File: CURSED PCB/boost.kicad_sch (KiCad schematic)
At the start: 6 parts, among them U11 TPS61046YFFR

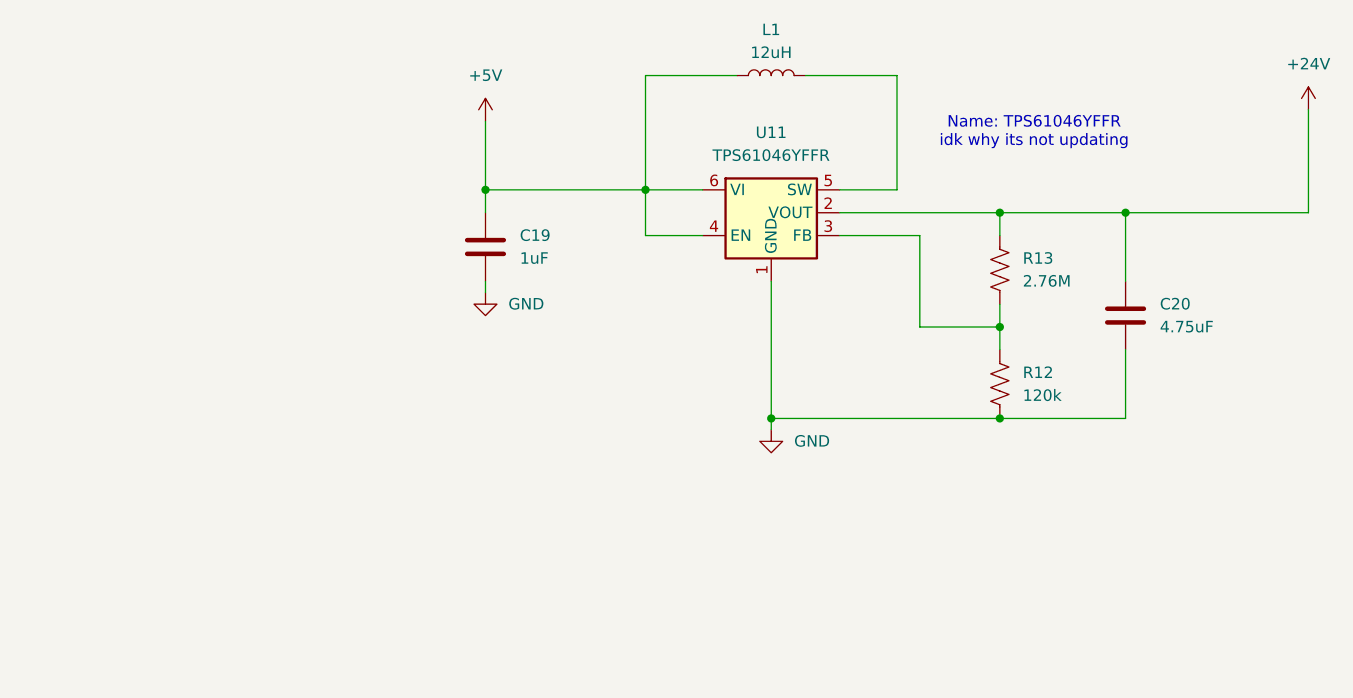
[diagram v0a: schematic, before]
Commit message: updated booster
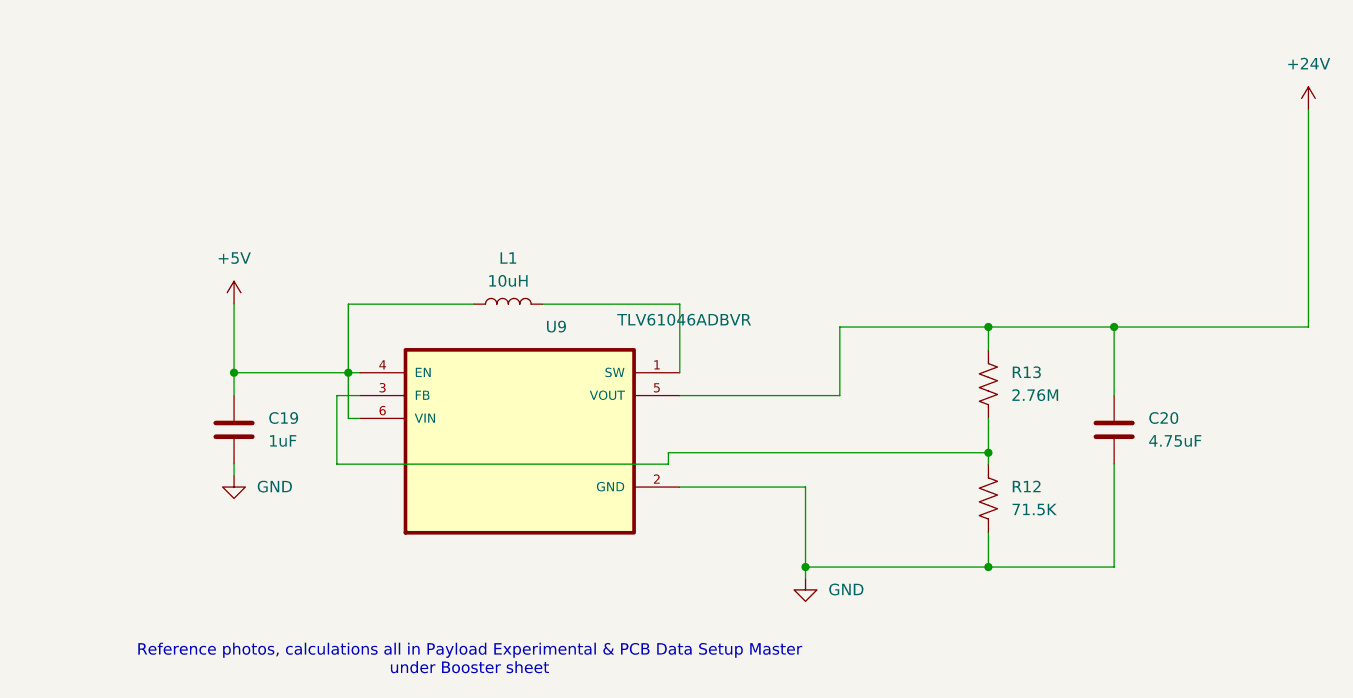
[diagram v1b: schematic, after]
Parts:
- removed U11: TPS61046YFFR, Package_SON:WSON-6-1EP_2x2mm_P0.65mm_EP1x1.6mm, symbol Regulator_Switching:TPS610995DRV
- added U9: TLV61046ADBVR, TLV61046A:SOT95P280X145-6N, symbol TLV61046A:TLV61046ADBVR
- L1: value 12uH -> 10uH
- R12: value 120k -> 71.5K
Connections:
- net +24V: now also U9.5 (VOUT)
- net +5V: now also U9.4 (EN), U9.6 (VIN)
- net GND: now also U9.2 (GND)
- net at L1.2: now also U9.1 (SW)
- net at R12.2, R13.1: now also U9.3 (FB)
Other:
- note added: "Reference photos, calculations all in Payload Experimental & PCB Data Setup Master under Booster sheet"
- note removed: "Name: TPS61046YFFR idk why its not updating"
- moved on the sheet: C19, C20, L1, R12, R13
